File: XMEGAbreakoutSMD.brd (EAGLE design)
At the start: 160 x 100 mm, 22 parts, among them IC1 XMEGA16A4A

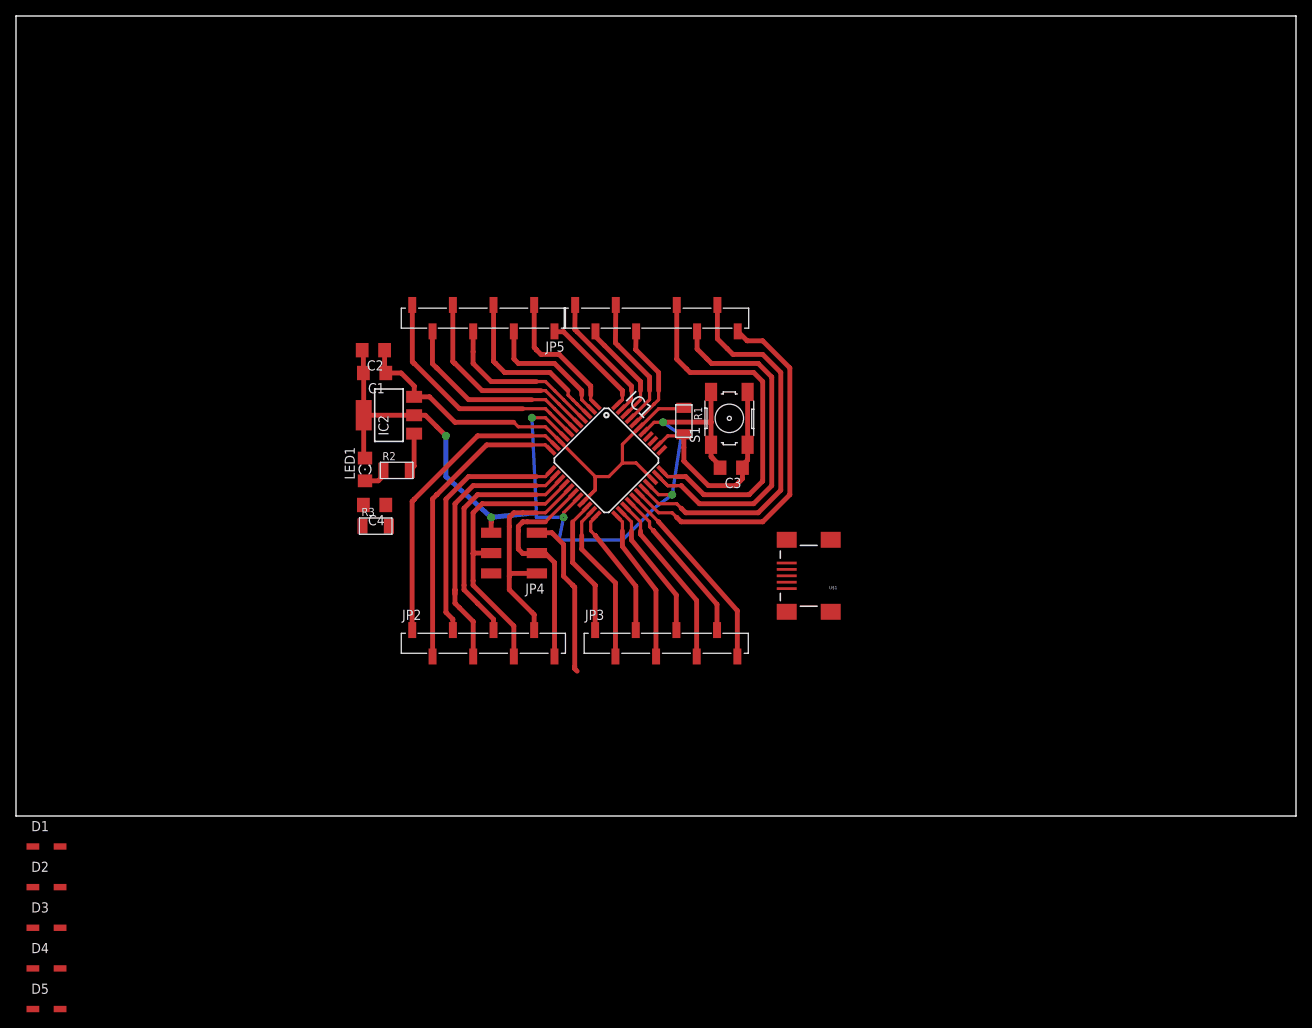
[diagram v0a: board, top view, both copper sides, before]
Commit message: smd breakout finished
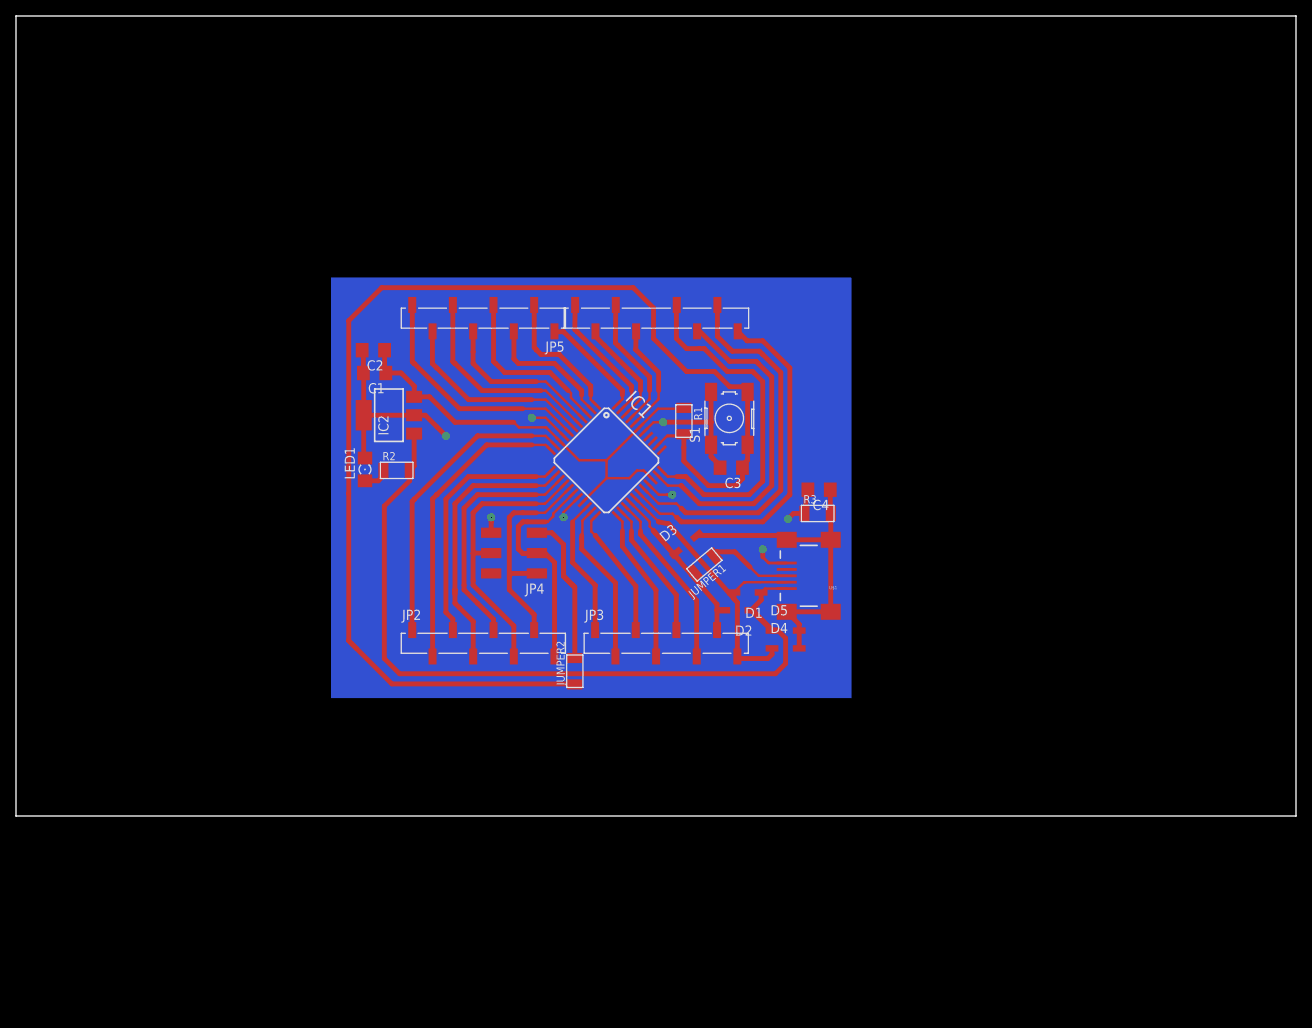
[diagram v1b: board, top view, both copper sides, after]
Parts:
- added JUMPER1, JUMPER2: 0, fab:R1206FAB
- IC1: value XMEGA16A4A -> XMEGA16A4; device atmel:TQFP44 -> atmel:TQFP44-FAB
- moved D5 103.8 mm to (96.2, 23.2)
- moved D4 100.7 mm to (96.2, 21.0)
- moved D3 93.3 mm to (83.8, 34.0), turned to 40 degrees
- moved D1 93.2 mm to (91.4, 27.9), turned to 180 degrees
- moved D2 93.0 mm to (90.2, 25.7), turned to 180 degrees
- moved C4 55.6 mm to (100.4, 40.8)
- moved R3 55.3 mm to (100.2, 37.8)
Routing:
- net RESET: track 47.8 -> 182.6 mm
- net VBUS: track 4.82 -> 99.9 mm
- net N$25: track 0.00 -> 44.7 mm
- net GND: track 121.3 -> 158.3 mm, vias 6 -> 8
- net D+: track 20.1 -> 37.3 mm
- net D-: track 24.8 -> 38.9 mm
- net PE2: track 46.3 -> 42.0 mm
- net PE3: track 47.9 -> 44.2 mm
- net VCC: track 64.0 -> 61.3 mm
- net MOSI: track 36.4 -> 35.3 mm

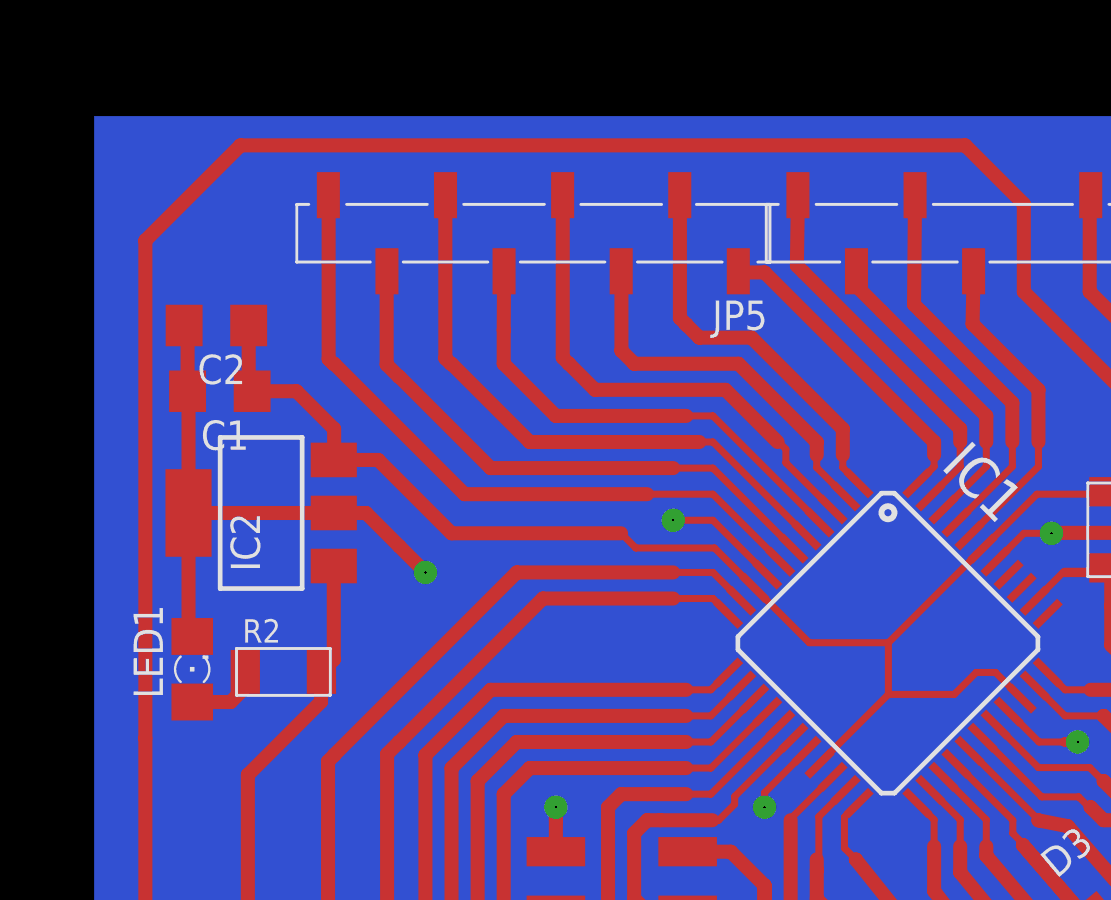
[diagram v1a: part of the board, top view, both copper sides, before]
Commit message: eagle layout finished
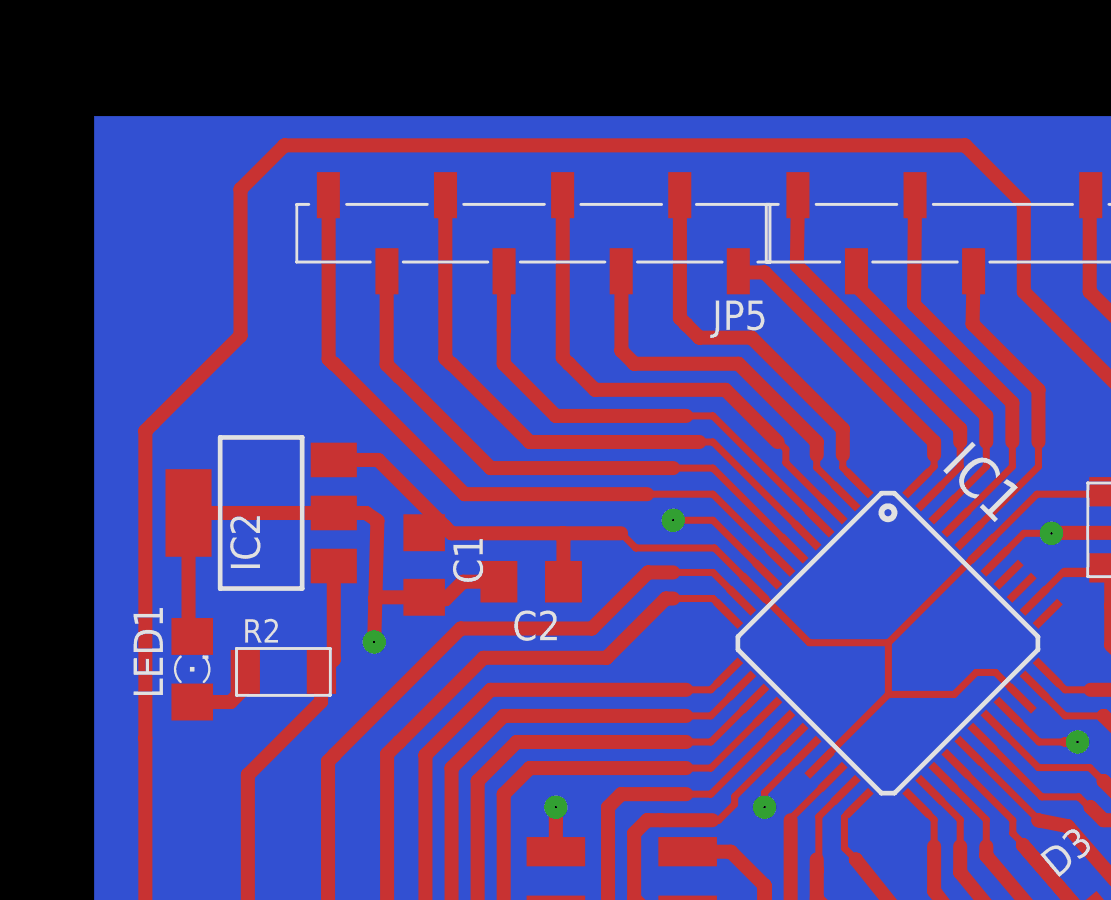
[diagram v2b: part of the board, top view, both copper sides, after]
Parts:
- moved C2 17.6 mm to (58.3, 47.1)
- moved C1 11.6 mm to (53.7, 47.8), turned to 270 degrees
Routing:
- net VCC: track 61.3 -> 56.0 mm
- net GND: track 158.3 -> 156.0 mm
- net RESET: track 182.6 -> 181.5 mm
